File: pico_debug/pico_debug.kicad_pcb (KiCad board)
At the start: 2 copper layers, 93 x 56 mm, 12 parts, among them J1 Conn_02x03_Counter_Clockwise, SW1 SW_SPST, SW2 SW_SPST, SW3 SW_SPST

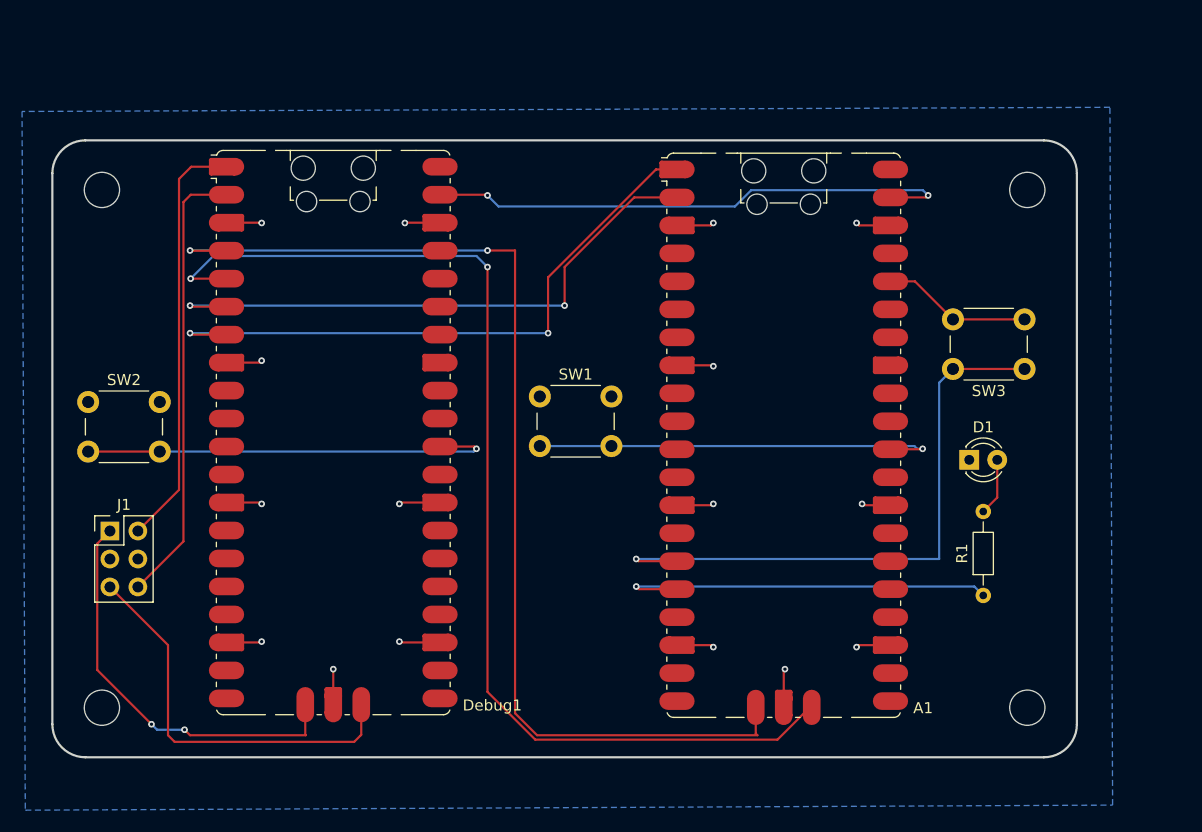
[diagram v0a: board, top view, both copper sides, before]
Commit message: v1 sent to pcbway
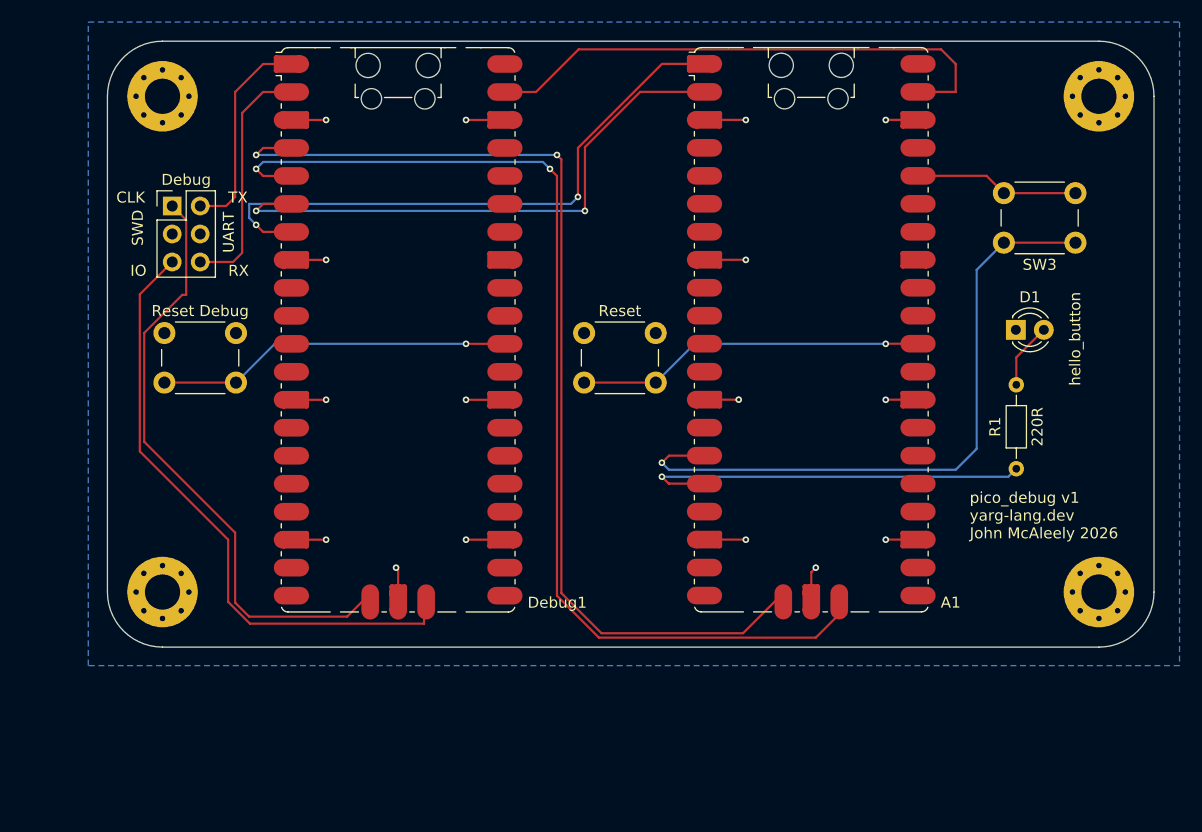
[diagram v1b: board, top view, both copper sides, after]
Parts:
- removed J1: Conn_02x03_Counter_Clockwise, Connector_PinHeader_2.54mm:PinHeader_2x03_P2.54mm_Vertical
- removed SW1, SW2: SW_SPST, Button_Switch_THT:SW_PUSH_6mm
- added Debug: Conn_02x03_Counter_Clockwise, Connector_PinHeader_2.54mm:PinHeader_2x03_P2.54mm_Vertical, F.Cu at (55.9, 65.0)
- added Reset: SW_SPST, Button_Switch_THT:SW_PUSH_6mm, F.Cu at (93.3, 76.5)
- added Reset Debug: SW_SPST, Button_Switch_THT:SW_PUSH_6mm, F.Cu at (55.2, 76.5)
- H1, H2, H3, H4: footprint MountingHole:MountingHole_3.2mm_M3 -> MountingHole:MountingHole_3.2mm_M3_Pad_Via
- moved H2 106.2 mm to (140.0, 55.0)
- moved H4 86.6 mm to (55.0, 100.0)
- moved D1 12.5 mm to (132.5, 76.2)
- moved SW3 12.4 mm to (137.9, 68.3)
- moved H3 12.3 mm to (140.0, 100.0)
- moved R1 11.9 mm to (132.5, 88.8)
- moved Debug1 11.0 mm to (76.4, 76.2)
- moved H1 10.1 mm to (55.0, 55.0)
- moved A1 9.90 mm to (113.9, 76.2)
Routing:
- net Net-(Debug1-SWDIO): track 37.2 -> 56.8 mm
- net Net-(Debug1-GPIO0): track 38.3 -> 19.2 mm
- net Net-(Debug1-GPIO1): track 40.8 -> 22.1 mm
- net Net-(Debug1-SWCLK): track 38.1 -> 55.4 mm, vias 2 -> 0
- net Net-(A1-SWCLK): track 101.0 -> 93.9 mm
- net Net-(Debug1-RUN): track 38.7 -> 32.4 mm
- net Net-(A1-RUN): track 37.8 -> 31.8 mm
- net Net-(A1-GPIO11): track 55.6 -> 60.0 mm
- net Net-(A1-SWDIO): track 103.2 -> 99.7 mm
- net Net-(A1-GPIO0): track 56.7 -> 54.8 mm
- net Net-(A1-GPIO1): track 53.7 -> 52.0 mm
- net +3.3V: track 13.6 -> 14.9 mm
- net Net-(A1-GPIO12): track 35.6 -> 36.6 mm
- net Net-(D1-A): track 5.22 -> 6.03 mm
- net VSYS: track 49.1 -> 49.0 mm, vias 2 -> 0
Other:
- board size 93 x 56 mm -> 95 x 55 mm
- board text added: "CLK"
- board text added: "IO"
- board text added: "RX"
- board text added: "SWD"
- board text added: "TX"
- board text added: "UART"
- board text added: "hello_button"
- board text added: "pico_debug v1 yarg-lang.dev John McAleely 2026"
